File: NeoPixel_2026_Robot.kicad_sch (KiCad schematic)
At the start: 1 part

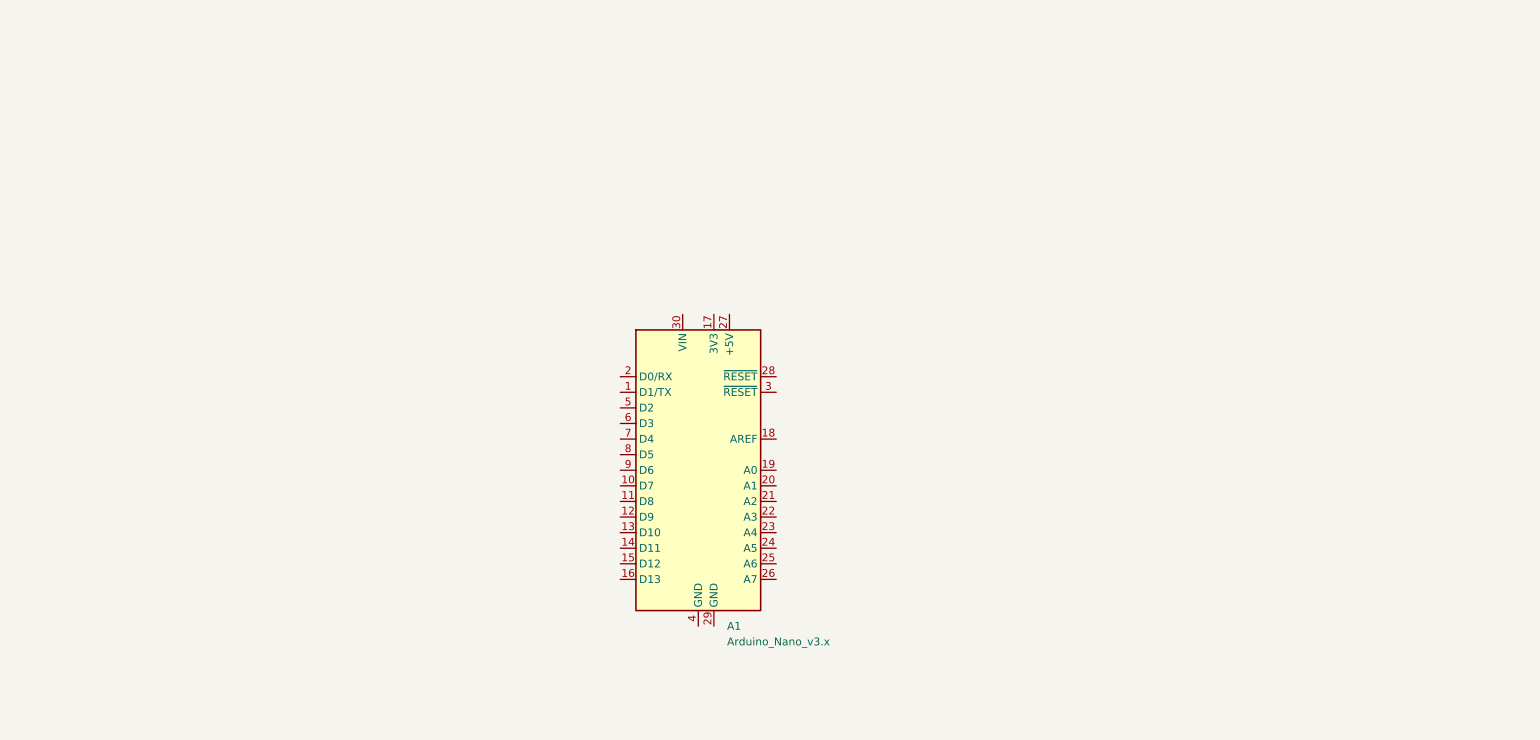
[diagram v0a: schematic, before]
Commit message: 回路図完成
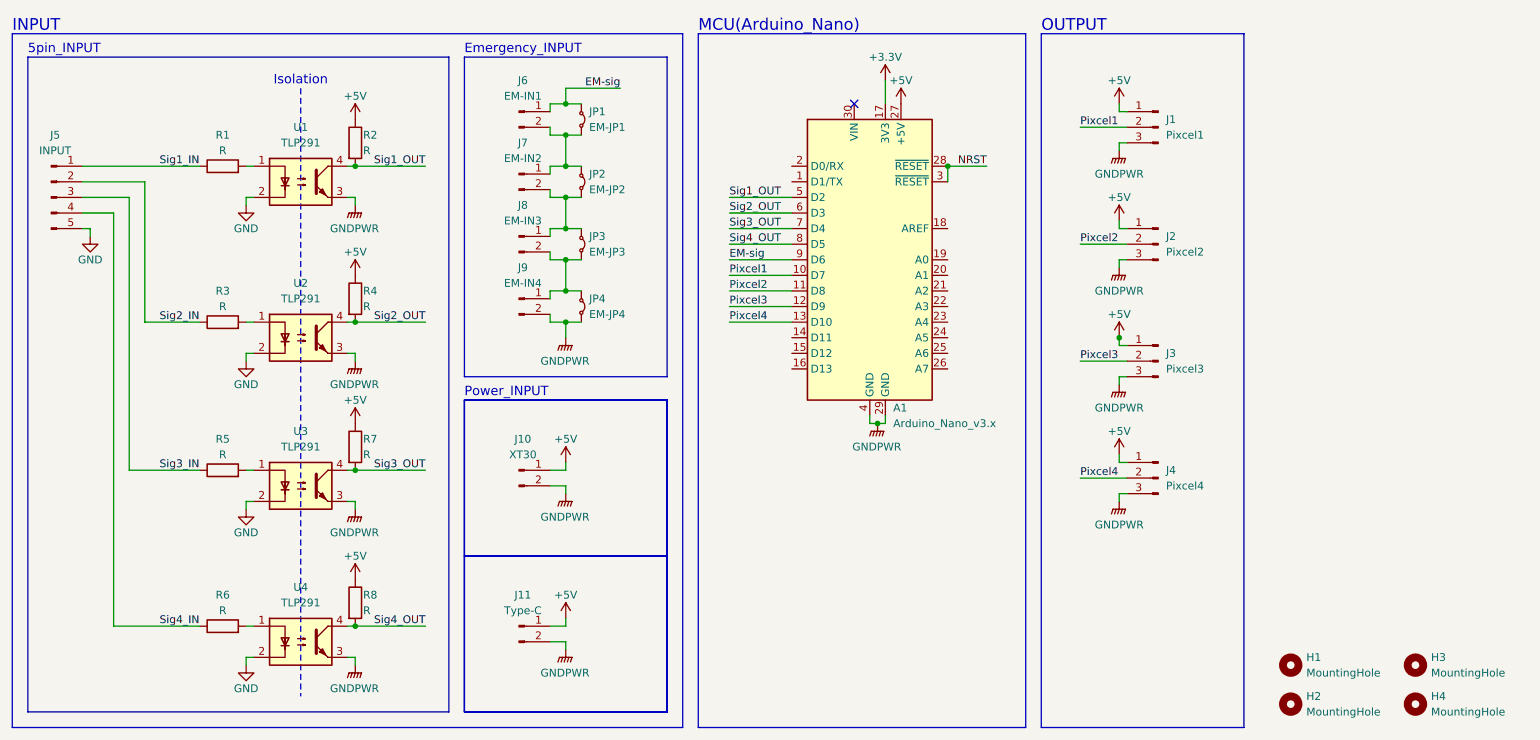
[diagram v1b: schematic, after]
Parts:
- added H1, H2, H3, H4: MountingHole, MountingHole:MountingHole_3.5mm_Pad, symbol Mechanical:MountingHole
- added J1: Pixcel1, Connector_JST:JST_XA_B03B-XASK-1_1x03_P2.50mm_Vertical, symbol Connector:Conn_01x03_Pin
- added J10: XT30, Connector_AMASS:AMASS_XT30PW-M_1x02_P2.50mm_Horizontal, symbol Connector:Conn_01x02_Pin
- added J11: Type-C, MyUSB_C:PowerOnlyUSB_C, symbol Connector:Conn_01x02_Pin
- added J2: Pixcel2, MountingHole:MountingHole_3.5mm_Pad, symbol Connector:Conn_01x03_Pin
- added J3: Pixcel3, MountingHole:MountingHole_3.5mm_Pad, symbol Connector:Conn_01x03_Pin
- added J4: Pixcel4, MountingHole:MountingHole_3.5mm_Pad, symbol Connector:Conn_01x03_Pin
- added J5: INPUT, Connector_JST:JST_XA_S05B-XASK-1_1x05_P2.50mm_Horizontal, symbol Connector:Conn_01x05_Pin
- added J6: EM-IN1, Connector_JST:JST_XA_B02B-XASK-1_1x02_P2.50mm_Vertical, symbol Connector:Conn_01x02_Pin
- added J7: EM-IN2, Connector_JST:JST_XA_B02B-XASK-1_1x02_P2.50mm_Vertical, symbol Connector:Conn_01x02_Pin
- added J8: EM-IN3, Connector_JST:JST_XA_B02B-XASK-1_1x02_P2.50mm_Vertical, symbol Connector:Conn_01x02_Pin
- added J9: EM-IN4, Connector_JST:JST_XA_B02B-XASK-1_1x02_P2.50mm_Vertical, symbol Connector:Conn_01x02_Pin
- added JP1: EM-JP1, Connector_PinHeader_2.54mm:PinHeader_1x02_P2.54mm_Vertical, symbol Jumper:Jumper_2_Small_Bridged
- added JP2: EM-JP2, Connector_PinHeader_2.54mm:PinHeader_1x02_P2.54mm_Vertical, symbol Jumper:Jumper_2_Small_Bridged
- added JP3: EM-JP3, Connector_PinHeader_2.54mm:PinHeader_1x02_P2.54mm_Vertical, symbol Jumper:Jumper_2_Small_Bridged
- added JP4: EM-JP4, Connector_PinHeader_2.54mm:PinHeader_1x02_P2.54mm_Vertical, symbol Jumper:Jumper_2_Small_Bridged
- added R1, R2, R3, R4, R5, R6, R7, R8: R, Resistor_SMD:R_0603_1608Metric_Pad0.98x0.95mm_HandSolder, symbol Device:R
- added U1, U2, U3, U4: TLP291, Package_SO:SOIC-4_4.55x2.6mm_P1.27mm, symbol Isolator:TLP291
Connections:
- net Pixcel1: now reaches A1.10 (D7)
- net Pixcel1: now also J1.2 (Pin_2)
- net Pixcel2: now reaches A1.11 (D8)
- net Pixcel2: now also J2.2 (Pin_2)
- net Pixcel3: now reaches A1.12 (D9)
- net Pixcel3: now also J3.2 (Pin_2)
- net Pixcel4: now reaches A1.13 (D10)
- net Pixcel4: now also J4.2 (Pin_2)
- net +3.3V: now reaches A1.17 (3V3)
- net +5V: now reaches A1.27 (+5V)
- net +5V: now also J1.1 (Pin_1), J10.1 (Pin_1), J11.1 (Pin_1), J2.1 (Pin_1), J3.1 (Pin_1), J4.1 (Pin_1), R2.1, R4.1, R7.1, R8.1
- net NRST: now reaches A1.28 (~{RESET})
- net NRST: now also A1.3 (~{RESET})
- net GNDPWR: now reaches A1.29 (GND)
- net GNDPWR: now also A1.4 (GND), J1.3 (Pin_3), J10.2 (Pin_2), J11.2 (Pin_2), J2.3 (Pin_3), J3.3 (Pin_3), J4.3 (Pin_3), J9.2 (Pin_2), JP4.2 (B), U1.3, U2.3, U3.3, U4.3
- net Sig1_OUT: now reaches A1.5 (D2)
- net Sig1_OUT: now also R2.2, U1.4
- net Sig2_OUT: now reaches A1.6 (D3)
- net Sig2_OUT: now also R4.2, U2.4
- net Sig3_OUT: now reaches A1.7 (D4)
- net Sig3_OUT: now also R7.2, U3.4
- net Sig4_OUT: now reaches A1.8 (D5)
- net Sig4_OUT: now also R8.2, U4.4
- net EM-sig: now reaches A1.9 (D6)
- net EM-sig: now also J6.1 (Pin_1), JP1.1 (A)
- new net: R3.2, U2.1
- new net: R5.2, U3.1
- new net: R6.2, U4.1
- new net: J6.2 (Pin_2), J7.1 (Pin_1), JP1.2 (B), JP2.1 (A)
- new net: J7.2 (Pin_2), J8.1 (Pin_1), JP2.2 (B), JP3.1 (A)
- new net: J8.2 (Pin_2), J9.1 (Pin_1), JP3.2 (B), JP4.1 (A)
- new net: R1.2, U1.1
- new net GND: J5.5 (Pin_5), U1.2, U2.2, U3.2, U4.2
- new net Sig1_IN: J5.1 (Pin_1), R1.1
- new net Sig2_IN: J5.2 (Pin_2), R3.1
- new net Sig3_IN: J5.3 (Pin_3), R5.1
- new net Sig4_IN: J5.4 (Pin_4), R6.1
- no-connect marks 0 -> 1
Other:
- note added: "5pin_INPUT"
- note added: "Emergency_INPUT"
- note added: "INPUT"
- note added: "Isolation"
- note added: "MCU(Arduino_Nano)"
- note added: "OUTPUT"
- note added: "Power_INPUT"
- moved on the sheet: A1

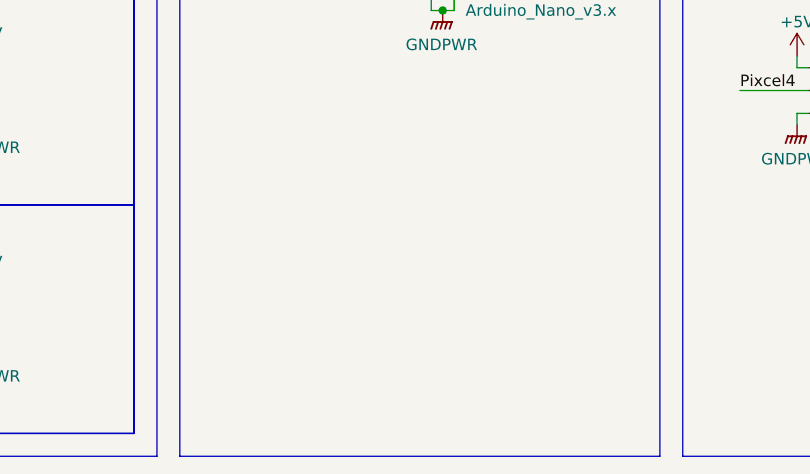
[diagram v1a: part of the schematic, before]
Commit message: おためし
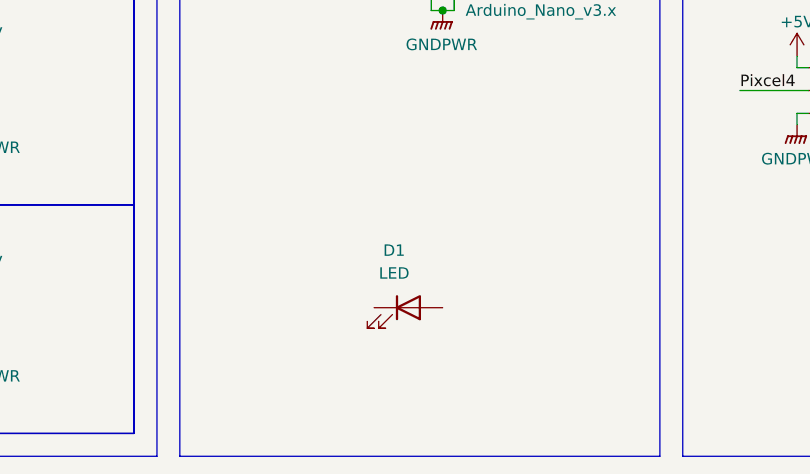
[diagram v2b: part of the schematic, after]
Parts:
- added D1: LED, symbol Device:LED
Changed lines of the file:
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@@
+	)
+	(symbol
+		(lib_id "Device:LED")
+		(at 151.13 113.03 0)
+		(unit 1)
+		(exclude_from_sim no)
+		(in_bom yes)
+		(on_board yes)
+		(dnp no)
+		(fields_autoplaced yes)
+		(property "Reference" "D1"
+			(at 149.5425 106.68 0)
+			(effects
+				(font
+					(size 1.27 1.27)
+				)
+			)
+		)
+		(property "Value" "LED"
+			(at 149.5425 109.22 0)
+			(effects
+				(font
+					(size 1.27 1.27)
+				)
+			)
+		)
+		(property "Footprint" ""
+			(at 151.13 113.03 0)
+			(effects
+				(font
+					(size 1.27 1.27)
+				)
+				(hide yes)
+			)
+		)
+		(property "Datasheet" "~"
+			(at 151.13 113.03 0)
+			(effects
+				(font
+					(size 1.27 1.27)
+				)
+				(hide yes)
+			)
+		)
+		(property "Description" "Light emitting diode"
+			(at 151.13 113.03 0)
+			(effects
+				(font
+					(size 1.27 1.27)
+				)
+				(hide yes)
+			)
+		)
+		(property "Sim.Pins" "1=K 2=A"
+			(at 151.13 113.03 0)
+			(effects
+				(font
+					(size 1.27 1.27)
+				)
+				(hide yes)
+			)
+		)
+		(pin "1"
+		)
+		(pin "2"
+		)
+		(instances
+			(project ""
+				(path "/874a96d0-c9ac-41c6-bdae-ae6107466332"
+					(reference "D1")
+					(unit 1)
+				)
+			)
+		)
 	)
 	(symbol

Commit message: windowsのほうで作ってたところまで手動復元
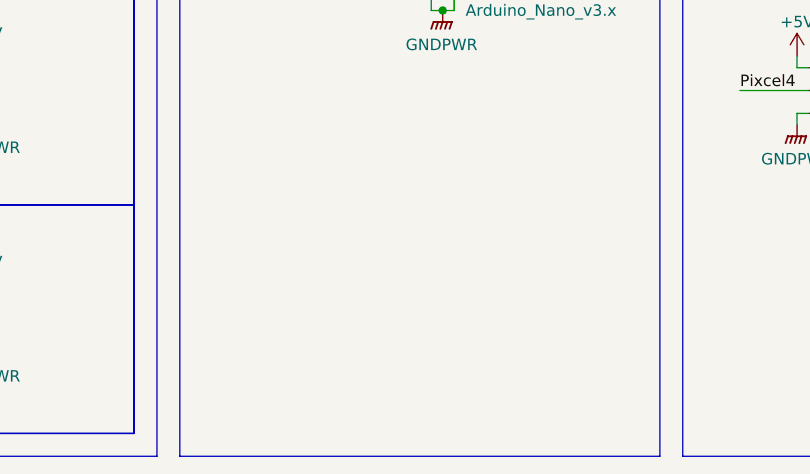
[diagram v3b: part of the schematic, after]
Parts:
- removed D1: LED, symbol Device:LED
- J11: footprint MyUSB_C:PowerOnlyUSB_C -> NeoPixcel_2026_Robot_Lib:PowerOnlyUSB_C
- J2, J3, J4: footprint MountingHole:MountingHole_3.5mm_Pad -> Connector_JST:JST_XA_B03B-XASK-1_1x03_P2.50mm_Vertical
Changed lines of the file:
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@@
 			)
 		)
-		(property "Footprint" "MountingHole:MountingHole_3.5mm_Pad"
+		(property "Footprint" "Connector_JST:JST_XA_B03B-XASK-1_1x03_P2.50mm_Vertical"
 			(at 200.66 88.9 0)
 			(effects
@@
 			)
 		)
-		(property "Footprint" "MountingHole:MountingHole_3.5mm_Pad"
+		(property "Footprint" "Connector_JST:JST_XA_B03B-XASK-1_1x03_P2.50mm_Vertical"
 			(at 200.66 69.85 0)
 			(effects
@@
 			)
 		)
-		(property "Footprint" "MyUSB_C:PowerOnlyUSB_C"
+		(property "Footprint" "NeoPixcel_2026_Robot_Lib:PowerOnlyUSB_C"
 			(at 96.52 113.03 0)
 			(effects
@@
 			)
 		)
-		(property "Footprint" "MountingHole:MountingHole_3.5mm_Pad"
+		(property "Footprint" "Connector_JST:JST_XA_B03B-XASK-1_1x03_P2.50mm_Vertical"
 			(at 200.66 50.8 0)
 			(effects
@@
 					(unit 1)
 				)
-			)
-		)
-	)
-	(symbol
-		(lib_id "Device:LED")
-		(at 151.13 113.03 0)
-		(unit 1)
-		(exclude_from_sim no)
-		(in_bom yes)
-		(on_board yes)
-		(dnp no)
-		(fields_autoplaced yes)
-		(property "Reference" "D1"
-			(at 149.5425 106.68 0)
-			(effects
-				(font
-					(size 1.27 1.27)
-				)
-			)
-		)
-		(property "Value" "LED"
-			(at 149.5425 109.22 0)
-			(effects
-				(font
-					(size 1.27 1.27)
-				)
-			)
-		)
-		(property "Footprint" ""
-			(at 151.13 113.03 0)
-			(effects
-				(font
-					(size 1.27 1.27)
-				)
-				(hide yes)
-			)
-		)
-		(property "Datasheet" "~"
-			(at 151.13 113.03 0)
-			(effects
-				(font
-					(size 1.27 1.27)
-				)
-				(hide yes)
-			)
-		)
-		(property "Description" "Light emitting diode"
-			(at 151.13 113.03 0)
-			(effects
-				(font
-					(size 1.27 1.27)
-				)
-				(hide yes)
-			)
-		)
-		(property "Sim.Pins" "1=K 2=A"
-			(at 151.13 113.03 0)
-			(effects
-				(font
-					(size 1.27 1.27)
-				)
-				(hide yes)
-			)
-		)
-		(pin "1"
-		)
-		(pin "2"
-		)
-		(instances
-			(project ""
-				(path "/874a96d0-c9ac-41c6-bdae-ae6107466332"
-					(reference "D1")
-					(unit 1)
-				)
